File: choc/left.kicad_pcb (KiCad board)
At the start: 2 copper layers, 118 x 92 mm, 87 parts, among them J1 USB_B_Micro, SW1 SW_Push, SW10 SW_Push, SW11 SW_Push, SW12 SW_Push, SW13 SW_Push, SW14 SW_Push, SW15 SW_Push, SW16 SW_Push, SW17 SW_Push, SW18 SW_Push, SW19 SW_Push, SW2 SW_Push, SW20 SW_Push, SW21 SW_Push, SW22 SW_Push, SW23 SW_Push, SW3 SW_Push, SW4 SW_Push, SW47 SW_Push, SW49 SW_Push, SW5 SW_Push, SW6 SW_Push, SW7 SW_Push, SW8 SW_Push, SW9 SW_Push, U1 ProMicro

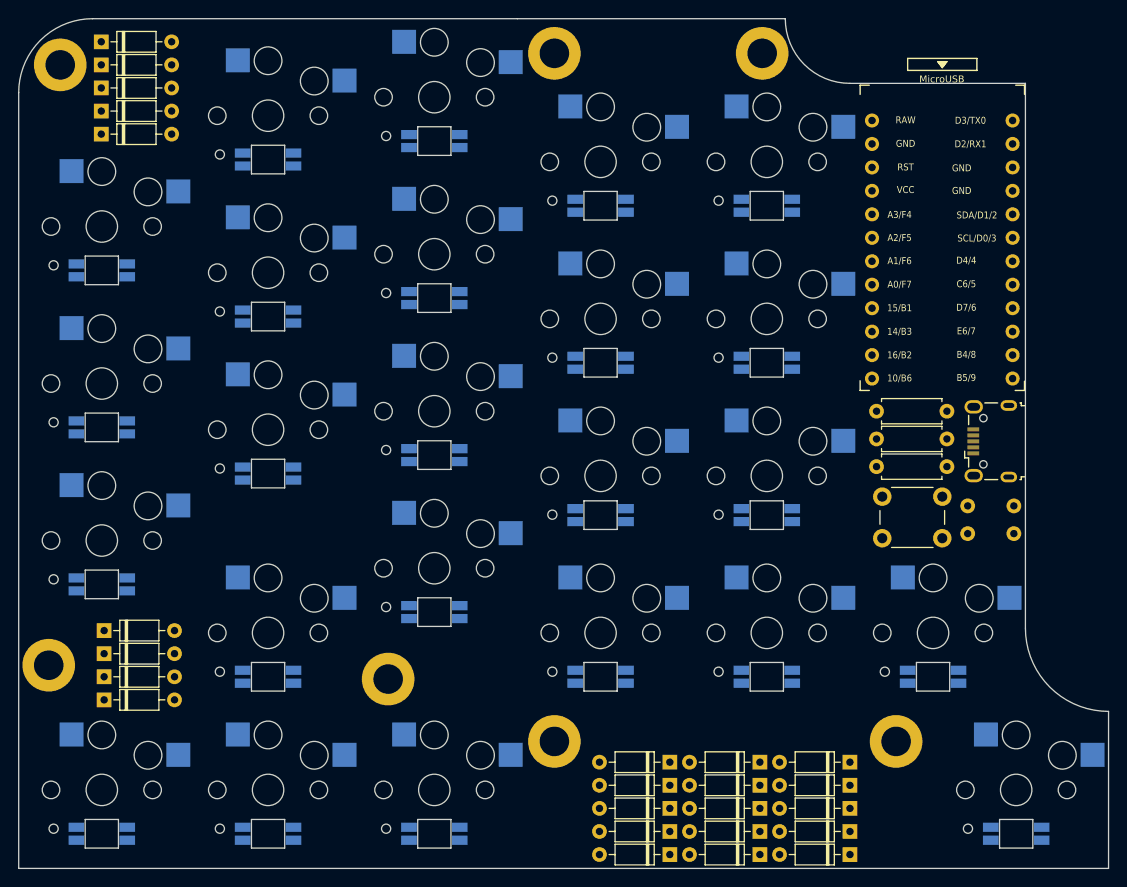
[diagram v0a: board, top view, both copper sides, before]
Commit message: progress
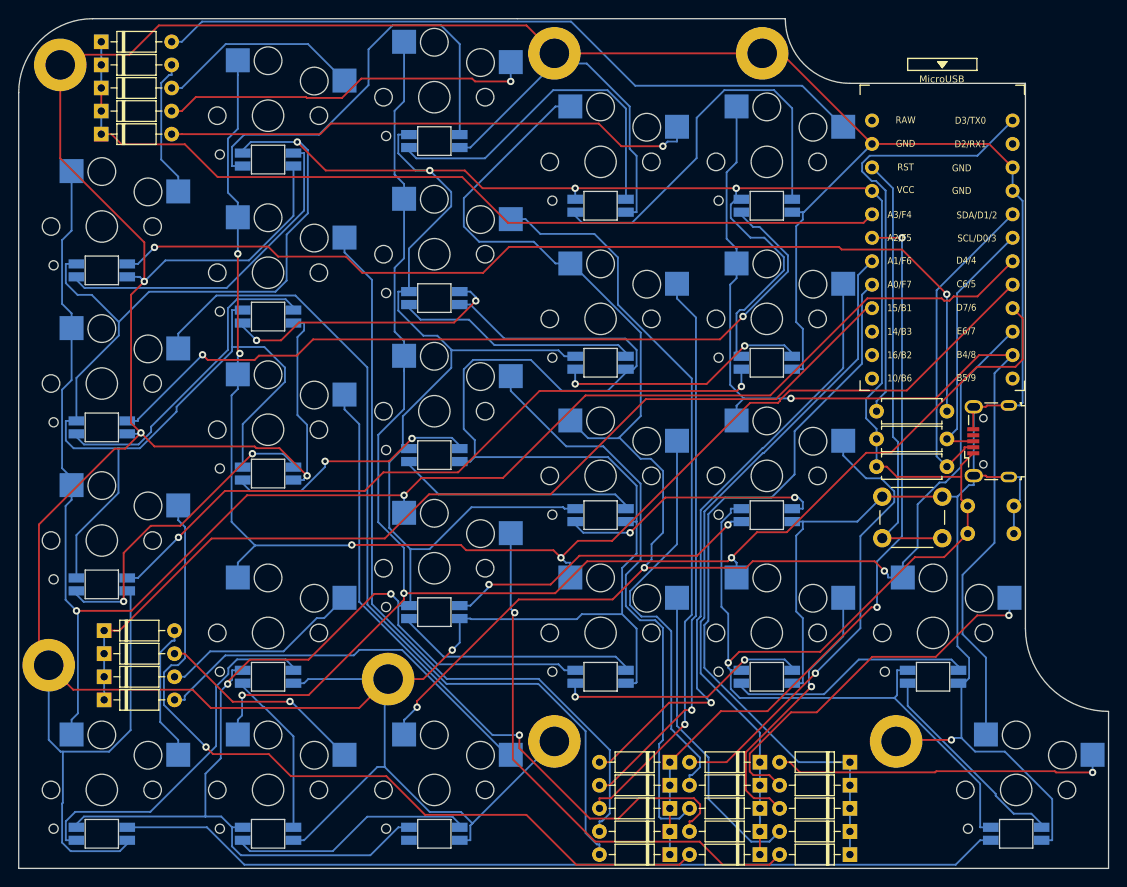
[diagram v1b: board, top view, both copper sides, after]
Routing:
- net GND: track 0.00 -> 753.6 mm, vias 0 -> 5
- net +5V: track 0.00 -> 578.4 mm, vias 0 -> 7
- net /lcol0: track 0.00 -> 183.0 mm, vias 0 -> 2
- net /lcol2: track 0.00 -> 176.5 mm, vias 0 -> 3
- net /lcol3: track 0.00 -> 174.6 mm, vias 0 -> 3
- net /lcol1: track 0.00 -> 156.9 mm, vias 0 -> 4
- net /lcol4: track 0.00 -> 111.5 mm, vias 0 -> 1
- net Net-(LED1-Pad4): track 0.00 -> 106.6 mm, vias 0 -> 2
- net /lrow4: track 0.00 -> 105.1 mm
- net /lrow0: track 0.00 -> 97.8 mm
- net Net-(LED23-Pad2): track 0.00 -> 96.3 mm
- net Net-(D2-Pad2): track 0.00 -> 96.1 mm
- net Net-(D3-Pad2): track 0.00 -> 87.8 mm, vias 0 -> 1
- net Net-(LED2-Pad4): track 0.00 -> 87.7 mm, vias 0 -> 2
- net /lrow1: track 0.00 -> 83.8 mm, vias 0 -> 2
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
